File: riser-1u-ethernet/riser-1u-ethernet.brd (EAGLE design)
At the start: 40 x 50 mm, 35 parts, among them IC1 ENC28J60SO, IC2 74HCT125D

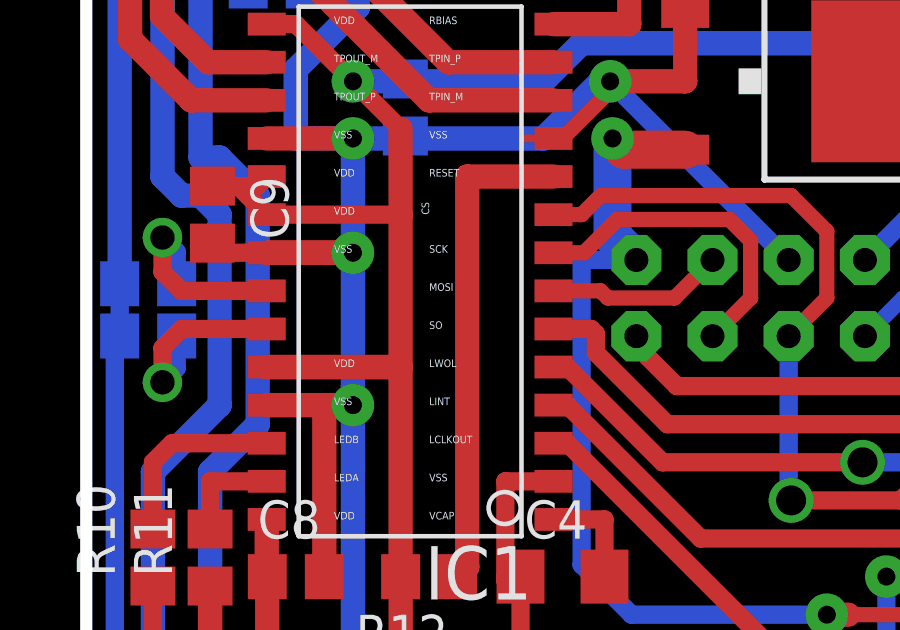
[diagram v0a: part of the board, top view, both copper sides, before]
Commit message: interim drop
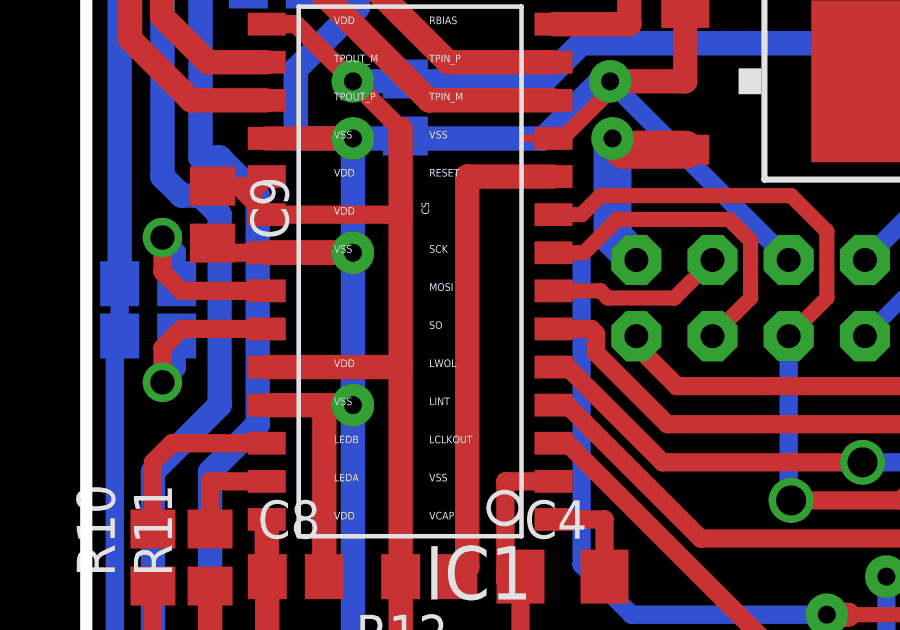
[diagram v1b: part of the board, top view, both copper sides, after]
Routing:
- net VCC: track 110.8 -> 104.5 mm
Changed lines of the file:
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@@
 <wire x1="6.985" y1="22.86" x2="6.015" y2="22.86" width="0.6096" layer="1"/>
 <wire x1="18.1769" y1="3.175" x2="24.6856" y2="3.175" width="0.6096" layer="16"/>
-<wire x1="10.4775" y1="11.43" x2="6.015" y2="11.43" width="0.8128" layer="1"/>
 <wire x1="10.4775" y1="11.43" x2="10.4775" y2="16.51" width="0.8128" layer="1"/>
 <wire x1="6.015" y1="4.465" x2="6.015" y2="6.35" width="0.8128" layer="1"/>
@@
 <wire x1="16.51" y1="4.8419" x2="18.1769" y2="3.175" width="0.6096" layer="16"/>
 <wire x1="16.51" y1="4.8419" x2="16.51" y2="15.0019" width="0.6096" layer="16"/>
-<wire x1="16.51" y1="15.0019" x2="18.3356" y2="15.0019" width="0.6096" layer="16"/>
 <wire x1="8.89" y1="20.955" x2="15.24" y2="20.955" width="0.8128" layer="16"/>
 <wire x1="15.24" y1="20.955" x2="16.51" y2="22.225" width="0.8128" layer="16"/>
